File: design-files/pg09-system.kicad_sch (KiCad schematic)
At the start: 10 parts, among them U101 MC6809E, U102 GAL22V10, U103 74AHCT245, U104 74AHCT245, U105 74AHCT245

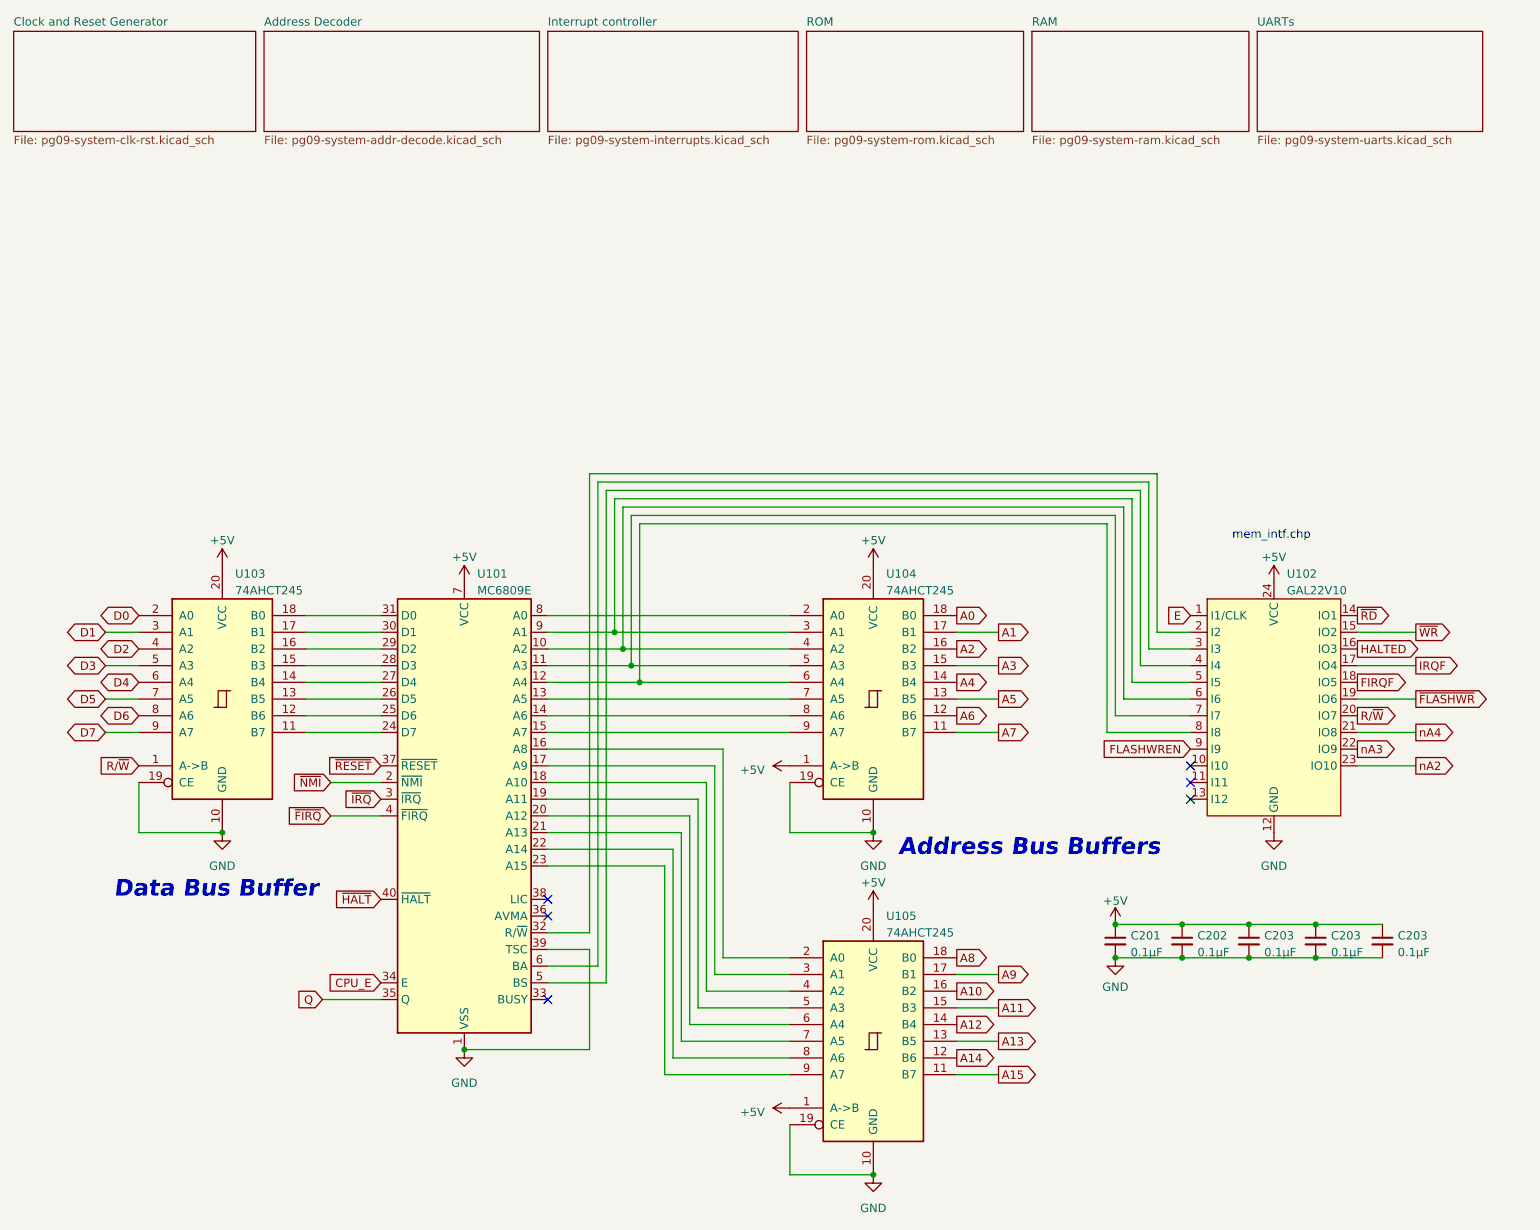
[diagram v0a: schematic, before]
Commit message: Connect the A5-A15 outputs of the 6809 directly to the inputs of the GALs that implement the address decoding logic.
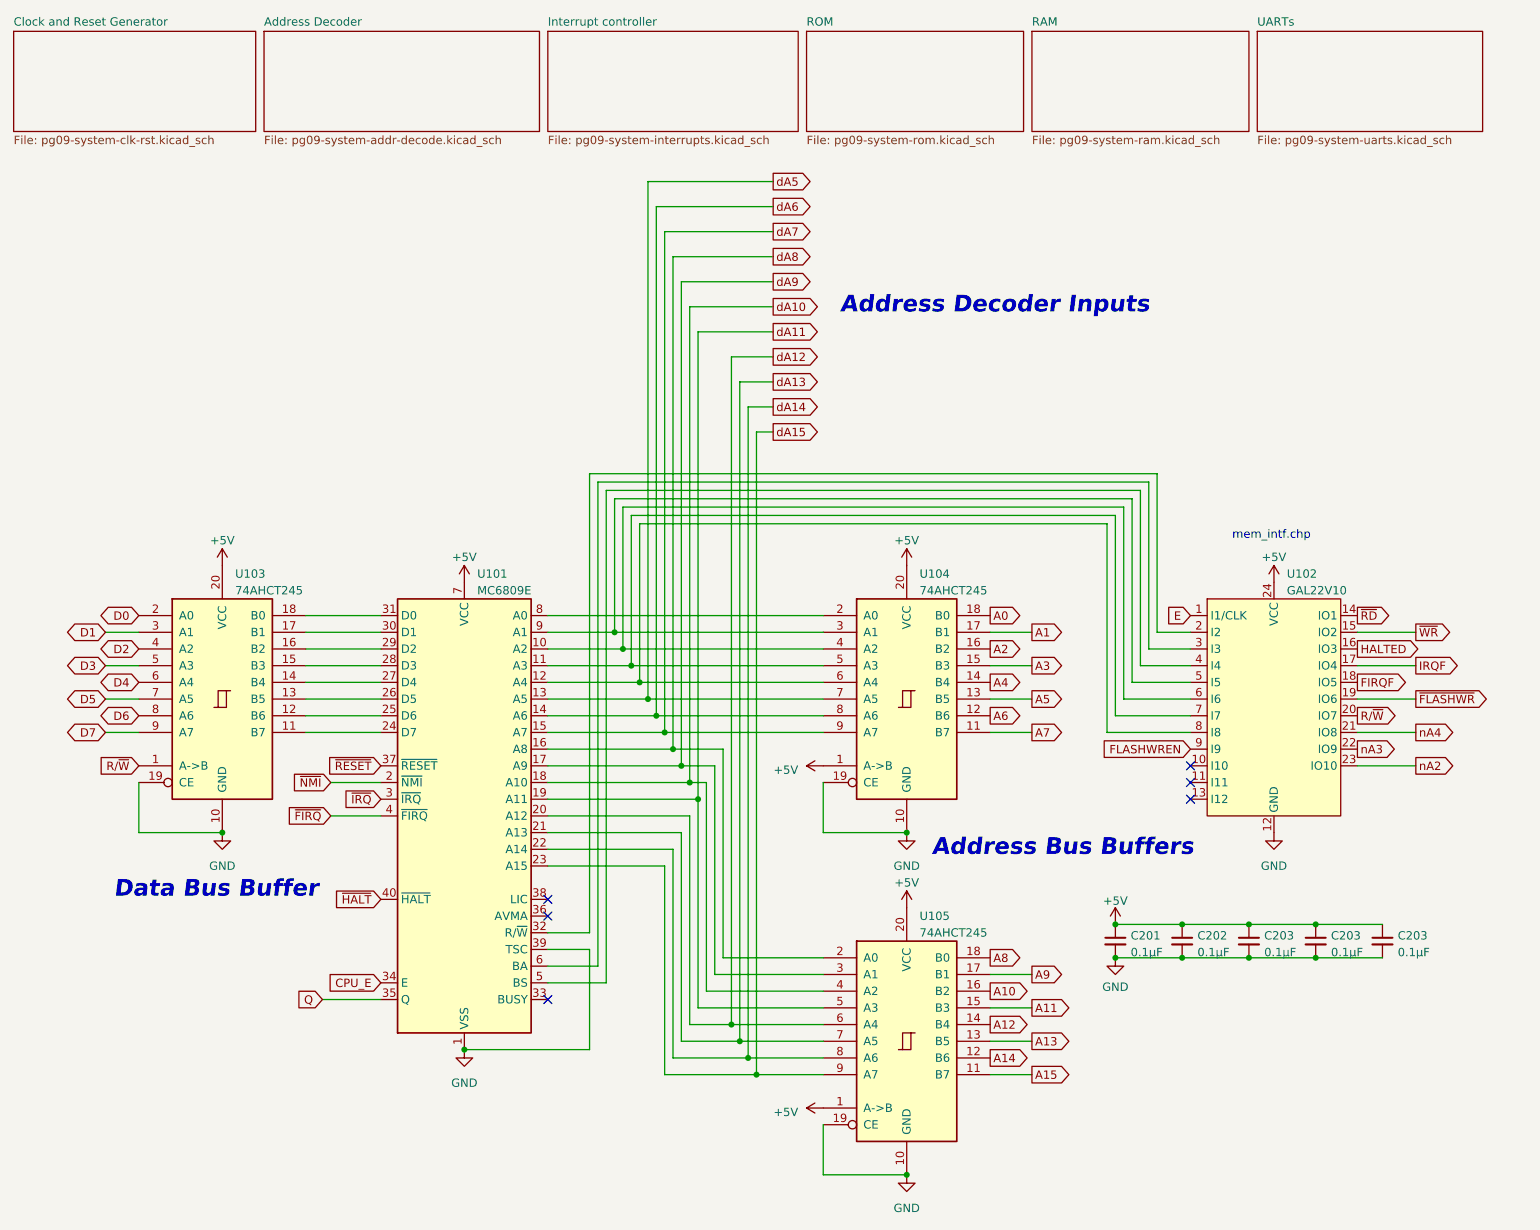
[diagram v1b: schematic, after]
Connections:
- net dA8: now reaches U101.16 (A8), U105.2 (A0)
- net dA9: now reaches U101.17 (A9), U105.3 (A1)
- net dA10: now reaches U101.18 (A10), U105.4 (A2)
- net dA11: now reaches U101.19 (A11), U105.5 (A3)
- net dA12: now reaches U101.20 (A12), U105.6 (A4)
- net dA13: now reaches U101.21 (A13), U105.7 (A5)
- net dA14: now reaches U101.22 (A14), U105.8 (A6)
- net dA15: now reaches U101.23 (A15), U105.9 (A7)
- net dA5: now reaches U101.13 (A5), U104.7 (A5)
- net dA6: now reaches U101.14 (A6), U104.8 (A6)
- net dA7: now reaches U101.15 (A7), U104.9 (A7)
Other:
- note added: "Address Decoder Inputs"
- moved on the sheet: U104, U105
